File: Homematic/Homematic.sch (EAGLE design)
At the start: 27 parts, among them IC1 3.3V, IC2 3.3V, P1 DF11-06-2DS, Q1 BS170

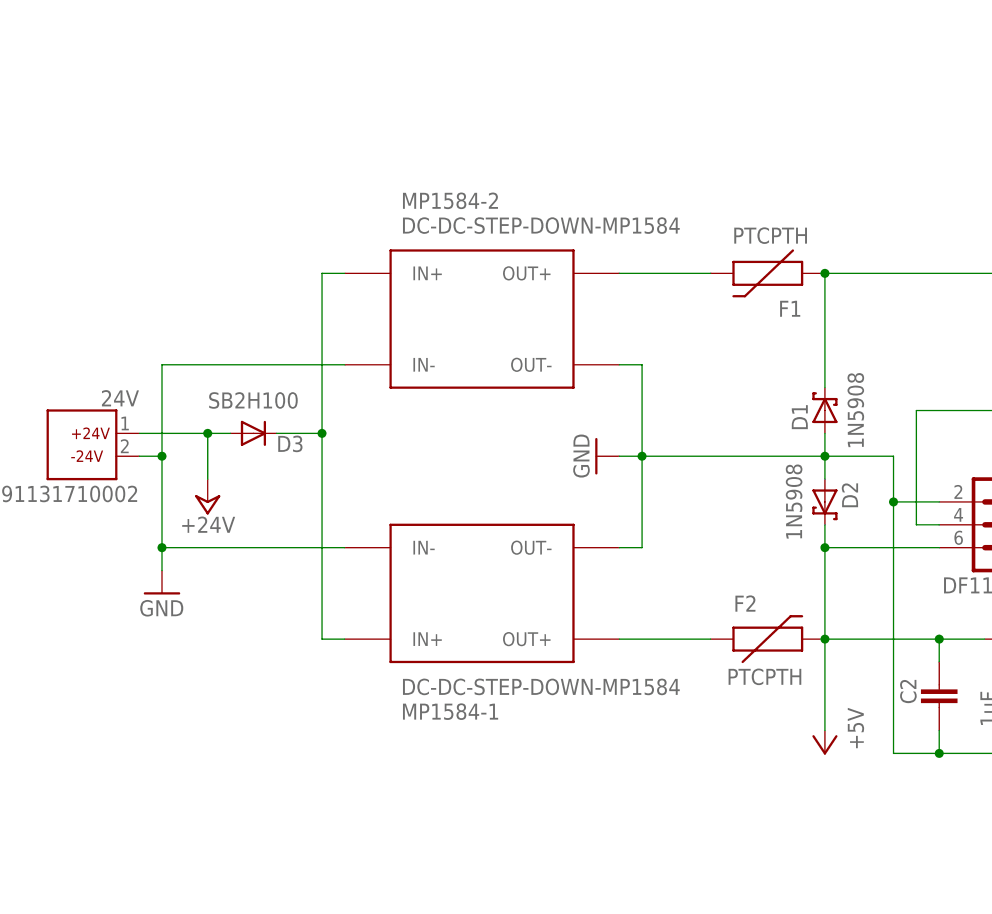
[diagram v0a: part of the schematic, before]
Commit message: Generate gerber files.
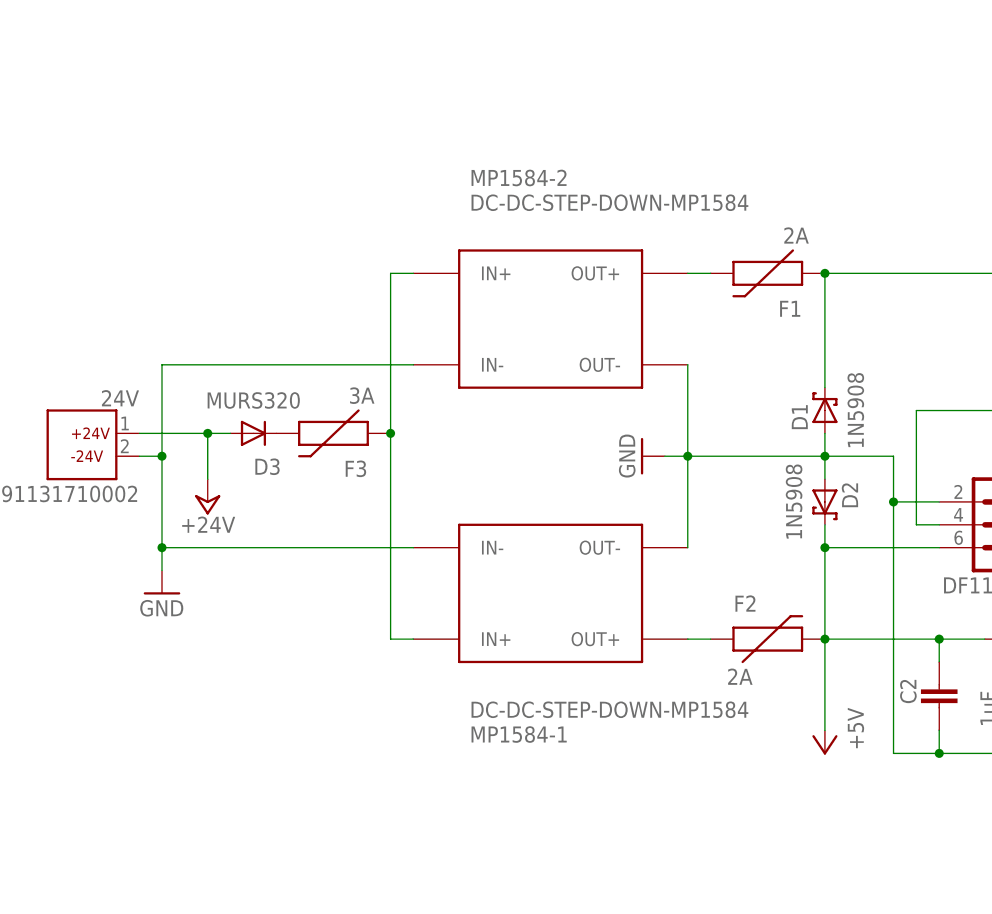
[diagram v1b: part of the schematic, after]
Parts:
- added F3: 3A, SparkFun-PowerIC:PTCPTH
- D3: value SB2H100 -> MURS320; device diode:DIODE-DO41-7.6 -> diode:DIODE-SMC
- F1, F2: value PTCPTH -> 2A
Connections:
- new net N$9: D3.C, F3.2
- net N$7: now also F3.1; no longer D3.C
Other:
- moved on the sheet: MP1584-1, MP1584-2
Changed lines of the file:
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@@
 <part name="D1" library="diode" deviceset="1N5908" device=""/>
 <part name="D2" library="diode" deviceset="1N5908" device=""/>
-<part name="F1" library="SparkFun-PowerIC" deviceset="PTC" device="PTH"/>
-<part name="F2" library="SparkFun-PowerIC" deviceset="PTC" device="PTH"/>
+<part name="F1" library="SparkFun-PowerIC" deviceset="PTC" device="PTH" value="2A"/>
+<part name="F2" library="SparkFun-PowerIC" deviceset="PTC" device="PTH" value="2A"/>
 <part name="GND1" library="supply1" deviceset="GND" device=""/>
 <part name="P+1" library="supply1" deviceset="+24V" device=""/>
@@
 <part name="MP1584-2" library="modules" deviceset="DC-DC-STEP-DOWN-MP1584" device=""/>
 <part name="MP1584-1" library="modules" deviceset="DC-DC-STEP-DOWN-MP1584" device=""/>
-<part name="D3" library="diode" deviceset="DIODE-" device="DO41-7.6" value="SB2H100"/>
+<part name="D3" library="diode" deviceset="DIODE-" device="SMC" value="MURS320"/>
 <part name="RXB8" library="modules" deviceset="WIRELESS-RXB8-5V" device=""/>
 <part name="GND3" library="supply1" deviceset="GND" device=""/>
@@
 <part name="C7" library="capacitor-wima" deviceset="C" device="2,5-3" value="100nF"/>
 <part name="GND7" library="supply1" deviceset="GND" device=""/>
+<part name="F3" library="SparkFun-PowerIC" deviceset="PTC" device="PTH" value="3A"/>
 </parts>
 <sheets>
@@
 <instance part="F1" gate="G$1" x="83.82" y="99.06" rot="R180"/>
 <instance part="F2" gate="G$1" x="81.28" y="58.42"/>
-<instance part="GND1" gate="1" x="63.5" y="78.74" rot="R270"/>
+<instance part="GND1" gate="1" x="68.58" y="78.74" rot="R270"/>
 <instance part="P+1" gate="1" x="20.32" y="73.66" smashed="yes" rot="R180">
 <attribute name="VALUE" x="20.32" y="71.12" size="1.778" layer="96" rot="R180" align="center"/>
@@
 <attribute name="MPN" x="193.04" y="17.78" size="1.778" layer="96" rot="MR270" display="off"/>
 </instance>
-<instance part="MP1584-2" gate="G$1" x="50.8" y="93.98"/>
-<instance part="MP1584-1" gate="G$1" x="50.8" y="63.5" rot="MR180"/>
+<instance part="MP1584-2" gate="G$1" x="58.42" y="93.98" smashed="yes">
+<attribute name="NAME" x="49.42" y="108.77" size="1.778" layer="95"/>
+<attribute name="VALUE" x="49.42" y="106.02" size="1.778" layer="96"/>
+</instance>
+<instance part="MP1584-1" gate="G$1" x="58.42" y="63.5" smashed="yes" rot="MR180">
+<attribute name="NAME" x="49.42" y="48.71" size="1.778" layer="95" rot="MR180"/>
+<attribute name="VALUE" x="49.42" y="51.46" size="1.778" layer="96" rot="MR180"/>
+</instance>
 <instance part="D3" gate="G$1" x="25.4" y="81.28" smashed="yes">
-<attribute name="NAME" x="27.94" y="79.2226" size="1.778" layer="95"/>
+<attribute name="NAME" x="25.4" y="76.6826" size="1.778" layer="95"/>
 <attribute name="VALUE" x="25.4" y="84.0486" size="1.778" layer="96" align="bottom-center"/>
 </instance>
@@
 </instance>
 <instance part="GND7" gate="1" x="177.8" y="58.42"/>
+<instance part="F3" gate="G$1" x="35.56" y="81.28" rot="R180"/>
 </instances>
 <busses>
@@
 <segment>
 <pinref part="GND1" gate="1" pin="GND"/>
-<wire x1="66.04" y1="78.74" x2="68.58" y2="78.74" width="0.1524" layer="91"/>
+<wire x1="71.12" y1="78.74" x2="73.66" y2="78.74" width="0.1524" layer="91"/>
 <pinref part="D2" gate="1" pin="A"/>
-<wire x1="68.58" y1="78.74" x2="88.9" y2="78.74" width="0.1524" layer="91"/>
+<wire x1="73.66" y1="78.74" x2="88.9" y2="78.74" width="0.1524" layer="91"/>
 <wire x1="88.9" y1="78.74" x2="88.9" y2="76.2" width="0.1524" layer="91"/>
 <pinref part="D1" gate="1" pin="A"/>
@@
 <junction x="96.52" y="73.66"/>
 <pinref part="MP1584-2" gate="G$1" pin="OUT-"/>
-<wire x1="66.04" y1="88.9" x2="68.58" y2="88.9" width="0.1524" layer="91"/>
-<wire x1="68.58" y1="88.9" x2="68.58" y2="78.74" width="0.1524" layer="91"/>
+<wire x1="73.66" y1="88.9" x2="73.66" y2="78.74" width="0.1524" layer="91"/>
 <pinref part="MP1584-1" gate="G$1" pin="OUT-"/>
-<wire x1="66.04" y1="68.58" x2="68.58" y2="68.58" width="0.1524" layer="91"/>
-<wire x1="68.58" y1="68.58" x2="68.58" y2="78.74" width="0.1524" layer="91"/>
-<junction x="68.58" y="78.74"/>
+<wire x1="73.66" y1="68.58" x2="73.66" y2="78.74" width="0.1524" layer="91"/>
+<junction x="73.66" y="78.74"/>
 <wire x1="96.52" y1="45.72" x2="101.6" y2="45.72" width="0.1524" layer="91"/>
 <pinref part="IC1" gate="1" pin="GND"/>
@@
 <wire x1="15.24" y1="68.58" x2="15.24" y2="66.04" width="0.1524" layer="91"/>
 <pinref part="MP1584-1" gate="G$1" pin="IN-"/>
-<wire x1="15.24" y1="68.58" x2="35.56" y2="68.58" width="0.1524" layer="91"/>
+<wire x1="15.24" y1="68.58" x2="43.18" y2="68.58" width="0.1524" layer="91"/>
 <junction x="15.24" y="68.58"/>
 <pinref part="GND3" gate="1" pin="GND"/>
@@
 <junction x="15.24" y="78.74"/>
 <pinref part="MP1584-2" gate="G$1" pin="IN-"/>
-<wire x1="15.24" y1="88.9" x2="35.56" y2="88.9" width="0.1524" layer="91"/>
+<wire x1="15.24" y1="88.9" x2="43.18" y2="88.9" width="0.1524" layer="91"/>
 </segment>
 <segment>
@@
 <pinref part="MP1584-2" gate="G$1" pin="OUT+"/>
 <pinref part="F1" gate="G$1" pin="2"/>
-<wire x1="66.04" y1="99.06" x2="76.2" y2="99.06" width="0.1524" layer="91"/>
+<wire x1="73.66" y1="99.06" x2="76.2" y2="99.06" width="0.1524" layer="91"/>
 </segment>
 </net>
@@
 <pinref part="MP1584-1" gate="G$1" pin="OUT+"/>
 <pinref part="F2" gate="G$1" pin="1"/>
-<wire x1="66.04" y1="58.42" x2="76.2" y2="58.42" width="0.1524" layer="91"/>
+<wire x1="73.66" y1="58.42" x2="76.2" y2="58.42" width="0.1524" layer="91"/>
 </segment>
 </net>
@@
 <net name="N$7" class="0">
 <segment>
+<pinref part="MP1584-2" gate="G$1" pin="IN+"/>
+<wire x1="40.64" y1="99.06" x2="43.18" y2="99.06" width="0.1524" layer="91"/>
+<wire x1="40.64" y1="99.06" x2="40.64" y2="81.28" width="0.1524" layer="91"/>
+<pinref part="MP1584-1" gate="G$1" pin="IN+"/>
+<wire x1="40.64" y1="81.28" x2="40.64" y2="58.42" width="0.1524" layer="91"/>
+<wire x1="40.64" y1="58.42" x2="43.18" y2="58.42" width="0.1524" layer="91"/>
+<pinref part="F3" gate="G$1" pin="1"/>
+<junction x="40.64" y="81.28"/>
+</segment>
+</net>
+<net name="N$9" class="0">
+<segment>
 <pinref part="D3" gate="G$1" pin="C"/>
-<wire x1="27.94" y1="81.28" x2="33.02" y2="81.28" width="0.1524" layer="91"/>
-<wire x1="33.02" y1="81.28" x2="33.02" y2="99.06" width="0.1524" layer="91"/>
-<pinref part="MP1584-2" gate="G$1" pin="IN+"/>
-<wire x1="33.02" y1="99.06" x2="35.56" y2="99.06" width="0.1524" layer="91"/>
-<wire x1="33.02" y1="81.28" x2="33.02" y2="58.42" width="0.1524" layer="91"/>
-<pinref part="MP1584-1" gate="G$1" pin="IN+"/>
-<wire x1="33.02" y1="58.42" x2="35.56" y2="58.42" width="0.1524" layer="91"/>
-<junction x="33.02" y="81.28"/>
-</segment>
-</net>
+<pinref part="F3" gate="G$1" pin="2"/>
+</segment>
+</net>
